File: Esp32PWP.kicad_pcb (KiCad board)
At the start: 2 copper layers, 57 x 33 mm, 37 parts, among them J1 HRO-TYPE-C-31-M-12, J2 Conn_02x03_Odd_Even, J3 Conn_01x02, Q1 MMBT3904, Q2 MMBT3904, SW1 SW_Push, U1 SRV05-4, U2 MC34063AD, U5 CP2102N-Axx-xQFN28

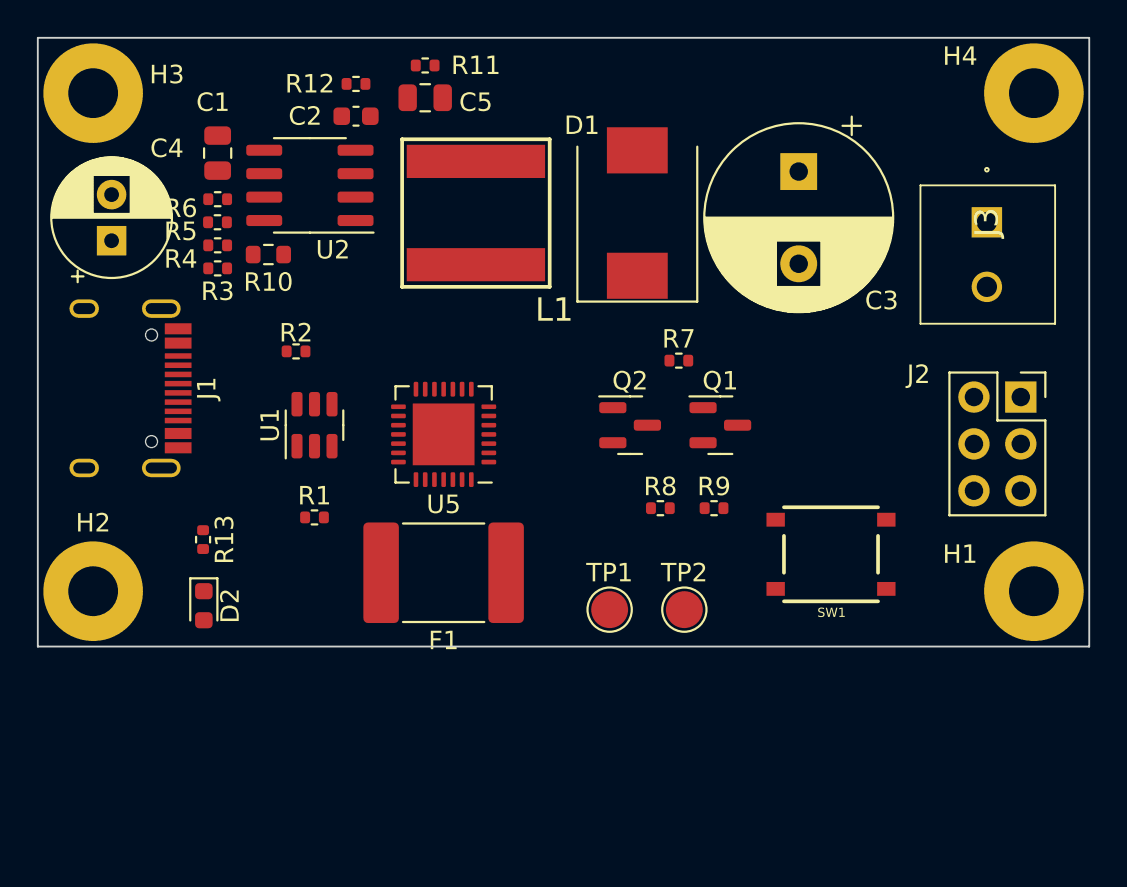
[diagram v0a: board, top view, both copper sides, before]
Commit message: feature creep
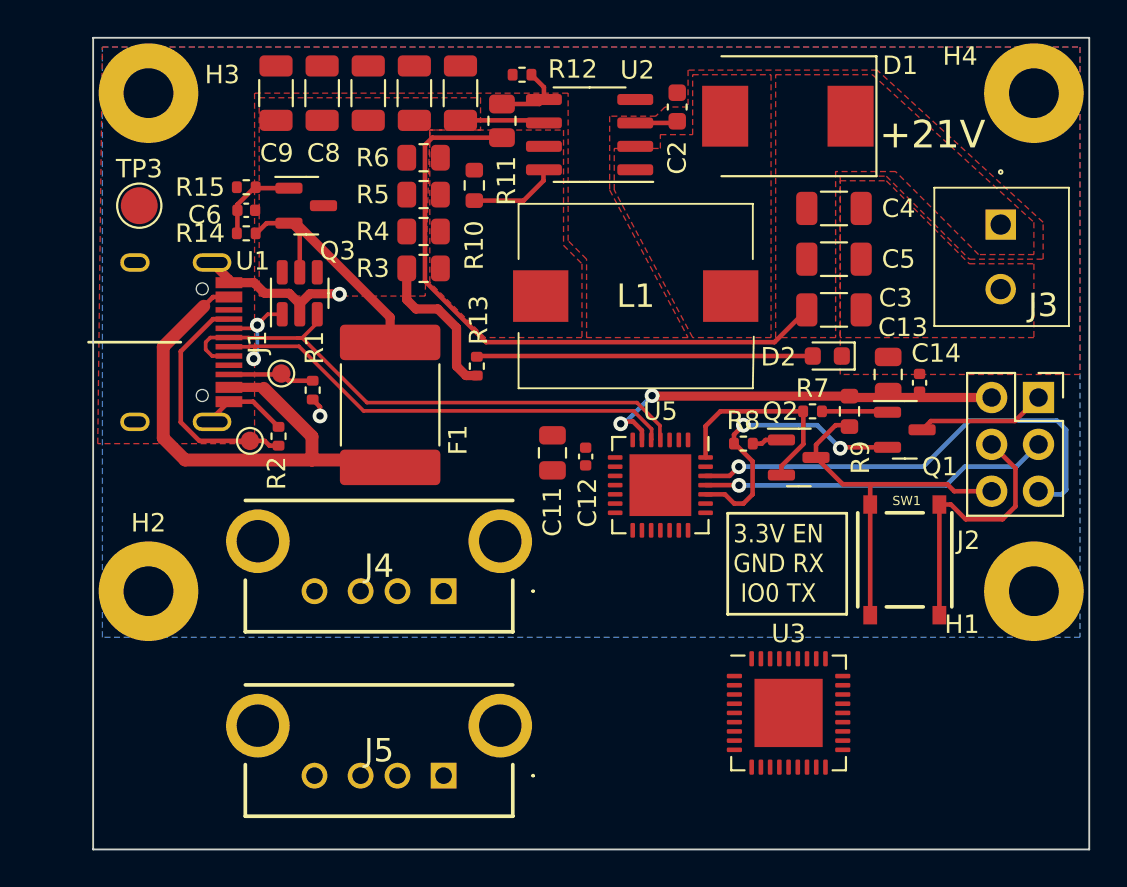
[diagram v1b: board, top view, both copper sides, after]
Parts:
- added C10: 22u/25V, Capacitor_SMD:C_1206_3216Metric, F.Cu at (129.9, 42.0)
- added C11: 2.2u, Capacitor_SMD:C_0805_2012Metric, F.Cu at (139.9, 61.5)
- added C12: 100n, Capacitor_SMD:C_0402_1005Metric, F.Cu at (141.7, 61.7)
- added C13: 2.2u, Capacitor_SMD:C_0805_2012Metric, F.Cu at (158.1, 57.2)
- added C14: 100n, Capacitor_SMD:C_0402_1005Metric, F.Cu at (159.8, 57.7)
- added C6: 100n, Capacitor_SMD:C_0402_1005Metric, F.Cu at (123.3, 48.4)
- added C7: 22u/25V, Capacitor_SMD:C_1206_3216Metric, F.Cu at (132.4, 42.0)
- added C8: 22u/25V, Capacitor_SMD:C_1206_3216Metric, F.Cu at (127.4, 42.0)
- added C9: 22u/25V, Capacitor_SMD:C_1206_3216Metric, F.Cu at (124.9, 42.0)
- added J4: USB_A, Local:UE27AE54100, F.Cu at (134.0, 69.0)
- added J5: USB_A, Local:UE27AE54100, F.Cu at (134.0, 79.0)
- added Q3: AO3401A, Package_TO_SOT_SMD:SOT-23, F.Cu at (126.5, 48.1)
- added R14: 100k, Resistor_SMD:R_0402_1005Metric, F.Cu at (123.3, 49.6)
- added R15: 4k7, Resistor_SMD:R_0402_1005Metric, F.Cu at (123.3, 47.1)
- added TP3: TestPoint, TestPoint:TestPoint_Pad_D2.0mm, F.Cu at (117.5, 48.1)
- added U3: USB2514B_Bi, Package_DFN_QFN:QFN-36-1EP_6x6mm_P0.5mm_EP3.7x3.7mm, F.Cu at (152.7, 75.6)
- C1, C5: value 10u/50V -> 22u/25V; footprint Capacitor_SMD:C_0805_2012Metric -> Capacitor_SMD:C_1206_3216Metric
- C2: value 680p -> 330p
- C3: value 330u/35V -> 22u/25V; footprint Capacitor_THT:CP_Radial_D10.0mm_P5.00mm -> Capacitor_SMD:C_1206_3216Metric
- C4: value 100u/35V -> 22u/25V; footprint Capacitor_THT:CP_Radial_D6.3mm_P2.50mm -> Capacitor_SMD:C_1206_3216Metric
- L1: value 68uH/1.2A -> 47uH/1.6A; footprint Local:NR8040T680M -> Local:PM3316680MRC
- R11, R3, R4, R5, R6: footprint Resistor_SMD:R_0402_1005Metric -> Resistor_SMD:R_0805_2012Metric
- R9: footprint Resistor_SMD:R_0402_1005Metric -> Resistor_SMD:R_0603_1608Metric
- TP1, TP2: footprint TestPoint:TestPoint_Pad_D2.0mm -> TestPoint:TestPoint_Pad_D1.0mm
- moved C4 39.2 mm to (155.2, 48.2), turned to 0 degrees
- moved D2 36.4 mm to (154.8, 56.2), turned to 180 degrees
- moved TP2 25.3 mm to (123.5, 60.9)
- moved C5 23.8 mm to (155.2, 51.0), turned to 0 degrees
- moved TP1 21.9 mm to (125.2, 57.2)
- moved R13 17.6 mm to (135.8, 56.8), turned to 90 degrees
- moved C2 17.4 mm to (146.7, 42.8), turned to 90 degrees
- moved U2 15.4 mm to (141.9, 44.2)
- moved C1 13.6 mm to (134.9, 42.0)
- moved U5 12.1 mm to (145.8, 63.2), turned to -90 degrees
- moved R10 11.8 mm to (135.7, 47.0), turned to -90 degrees
- moved R6 11.4 mm to (132.9, 45.5)
- moved R5 11.3 mm to (132.9, 47.5)
- moved R4 11.2 mm to (132.9, 49.5)
- moved R3 11.2 mm to (132.9, 51.5)
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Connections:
- C1 pad 1: VBUS -> VIN
- C4 pad 1: VBUS -> +24V
- R13 pad 1: VBUS -> VIN
- R3 pad 2: VBUS -> VIN
- R4 pad 2: VBUS -> VIN
- R5 pad 2: VBUS -> VIN
- R6 pad 2: VBUS -> VIN
- U2 pad 6: VBUS -> VIN
- U5 pad 7: +5V -> VIN
- U5 pad 8: +5V -> VIN
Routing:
- net +24V: track 0.00 -> 34.5 mm
- net USB_D-: track 0.00 -> 31.2 mm, vias 0 -> 2
- net USB_D+: track 0.00 -> 31.2 mm
- net Net-(F1-Pad2): track 0.00 -> 29.2 mm
- net GND: track 0.00 -> 29.2 mm, vias 0 -> 2
- net /USB2serial/TX: track 0.00 -> 25.9 mm, vias 0 -> 1
- net +3V3: track 0.00 -> 22.7 mm, vias 0 -> 2
- net /USB2serial/IO0: track 0.00 -> 20.4 mm
- net /USB2serial/RX: track 0.00 -> 19.0 mm, vias 0 -> 1
- net Net-(D2-Pad2): track 0.00 -> 18.2 mm
- net /USB2serial/RTS: track 0.00 -> 15.7 mm, vias 0 -> 2
- net VBUS: track 0.00 -> 14.7 mm
- net VIN: track 0.00 -> 13.0 mm
- net /CC1: track 0.00 -> 13.0 mm
- net /USB2serial/DTR: track 0.00 -> 11.3 mm
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- added copper zone on F.Cu, net +24V
- added copper zone on B.Cu, net GND
- added copper zone on F.Cu, net GND
- added copper zone on F.Cu, net Net-(D1-Pad2)
- added copper zone on F.Cu, net Net-(L1-Pad1)
- added copper zone on F.Cu, net VIN
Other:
- board size 57 x 33 mm -> 54 x 44 mm
- board text added: "+21V"
- board text added: "3.3V EN GND RX IO0 TX"

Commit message: ready for JLCPCB
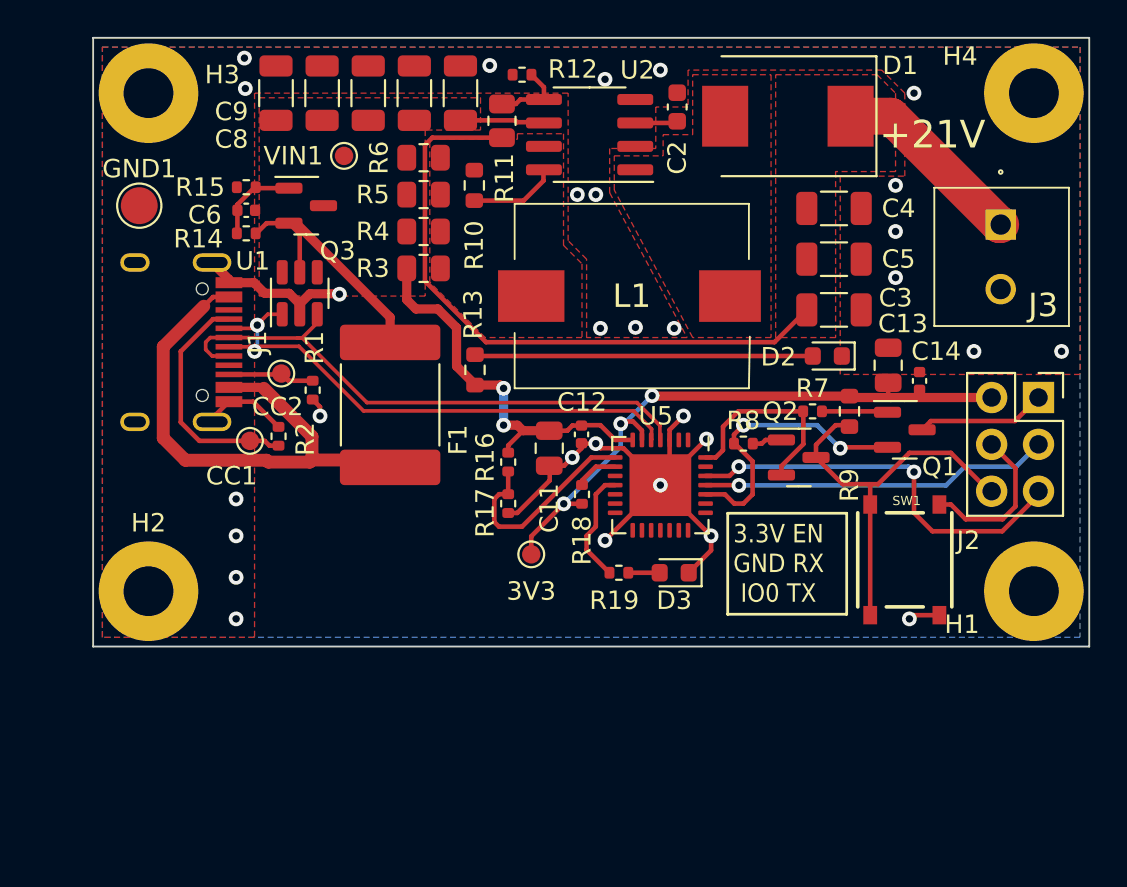
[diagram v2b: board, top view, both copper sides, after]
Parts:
- removed J4, J5: USB_A, Local:UE27AE54100
- removed U3: USB2514B_Bi, Package_DFN_QFN:QFN-36-1EP_6x6mm_P0.5mm_EP3.7x3.7mm
- added 3V3: TestPoint, TestPoint:TestPoint_Pad_D1.0mm, F.Cu at (138.8, 67.0)
- added D3: LED_GREEN, LED_SMD:LED_0603_1608Metric, F.Cu at (146.5, 68.0)
- added R16: 22k, Resistor_SMD:R_0402_1005Metric, F.Cu at (137.5, 62.0)
- added R17: 47k, Resistor_SMD:R_0402_1005Metric, F.Cu at (137.5, 64.2)
- added R18: 4k7, Resistor_SMD:R_0402_1005Metric, F.Cu at (141.5, 63.8)
- added R19: 220R, Resistor_SMD:R_0402_1005Metric, F.Cu at (143.5, 68.0)
- added VIN1: TestPoint, TestPoint:TestPoint_Pad_D1.0mm, F.Cu at (128.6, 45.4)
- R13: footprint Resistor_SMD:R_0402_1005Metric -> Resistor_SMD:R_0603_1608Metric
- moved C12 1.22 mm to (141.5, 60.5)
- moved C13 0.50 mm to (158.1, 56.8)
- moved C11 0.31 mm to (139.7, 61.2)
- moved R13 0.22 mm to (135.7, 57.0)
- moved L1 0.21 mm to (144.2, 53.0)
- moved C14 0.10 mm to (159.8, 57.6)
- renumbered TP2 to CC1, TP1 to CC2, TP3 to GND1
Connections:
- U5 pad 11: unconnected-(U5-Pad11) -> Net-(R19-Pad1)
- U5 pad 8: VIN -> Net-(R16-Pad2)
- U5 pad 9: unconnected-(U5-Pad9) -> Net-(R18-Pad2)
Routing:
- net GND: track 29.2 -> 54.7 mm, vias 2 -> 30
- net VIN: track 13.0 -> 25.9 mm, vias 0 -> 2
- net Net-(R16-Pad2): track 0.00 -> 11.5 mm
- net +3V3: track 22.7 -> 33.7 mm, vias 2 -> 3
- net +24V: track 34.5 -> 45.1 mm
- net Net-(R19-Pad1): track 0.00 -> 6.23 mm
- net /USB2serial/TX: track 25.9 -> 22.0 mm, vias 1 -> 2
- net Net-(R18-Pad2): track 0.00 -> 2.35 mm
- net Net-(D3-Pad2): track 0.00 -> 1.70 mm
- net /USB2serial/IO0: track 20.4 -> 21.8 mm
- net USB_D-: track 31.2 -> 30.4 mm
- net VBUS: track 14.7 -> 13.9 mm
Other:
- board size 54 x 44 mm -> 54 x 33 mm
